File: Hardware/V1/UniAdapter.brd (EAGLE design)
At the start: 40 x 20.9 mm, 19 parts, among them IC1 LD1117S33TR, U1 STM32F072CBT6, U2 SN65HVD232D, X1 CAN Bus

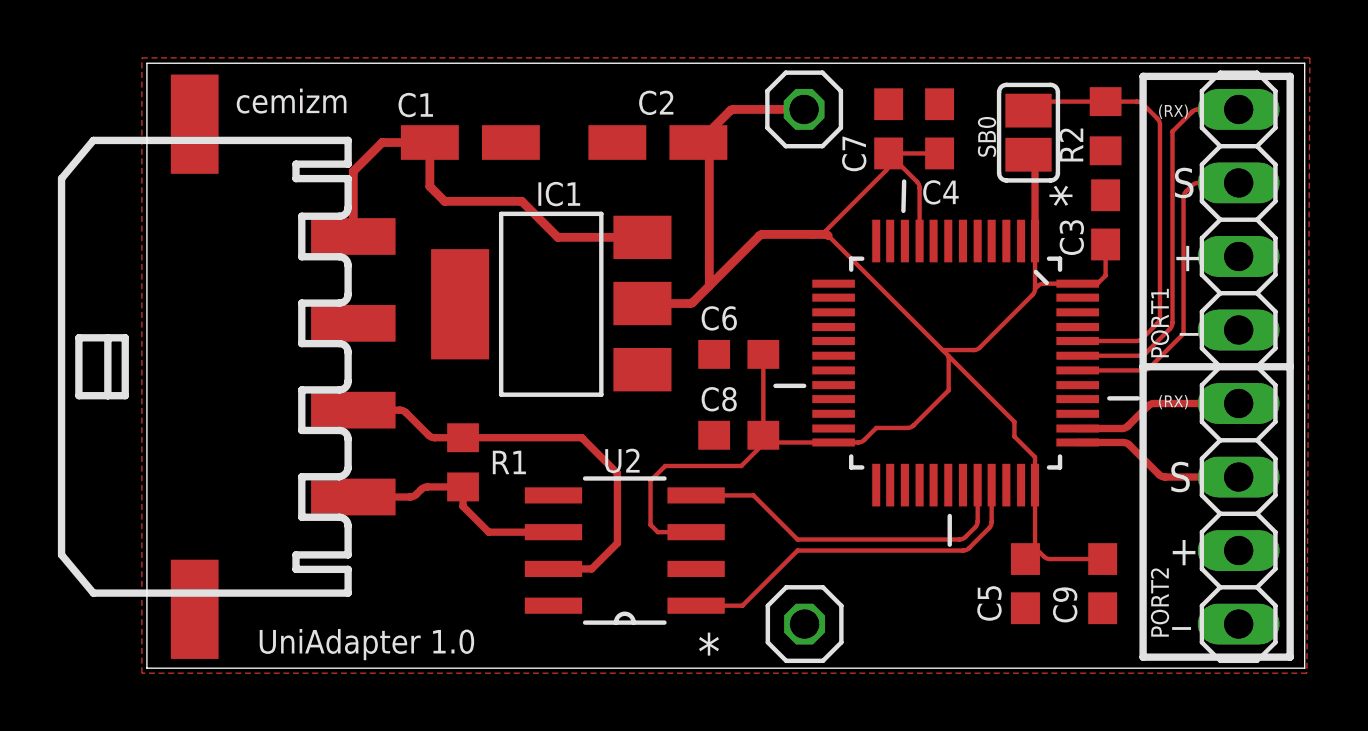
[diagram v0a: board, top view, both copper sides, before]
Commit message: [HW] UniAdapter 1.1
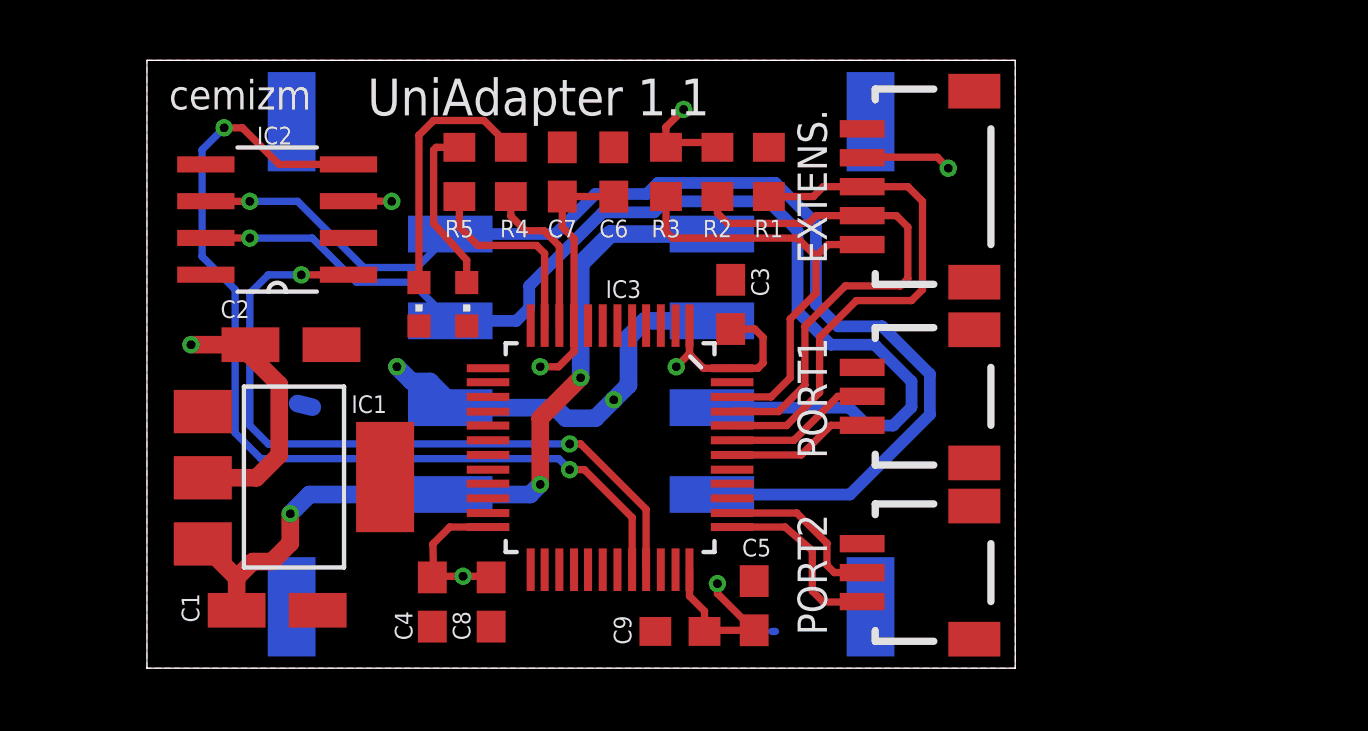
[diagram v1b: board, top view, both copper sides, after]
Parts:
- removed JP1: (no value), pinhead:1X08
- removed JP2, JP3: (no value), pinhead:1X01
- removed SB0: (no value), jumper:SJ
- removed U1: STM32F072CBT6, STM32F0:QFP50P900X900X160-48N
- removed U2: SN65HVD232D, texas:SOIC127P600X175-8N
- added EXTENS.: SM05B-SRSS-TB, con-jst2:SM05B-SRSS-TB
- added IC2: SN65HVD232D, texas:SOIC127P600X175-8N
- added IC3: STM32F072CBT6, STM32F0:LQFP48
- added LED_GREEN, LED_RED: (no value), led:CHIPLED_0603
- added PORT1, PORT2: SM03B-SRSS-TB, con-jst2:SM03B-SRSS-TB
- added R3: 1.8K, rcl:R0603
- added R4, R5: 55Ohm, rcl:R0603
- added X2: CAN Bus, con-molex-micro-fit-3_0:43650-0412
- C4: value 10nF -> 100nF
- C6: value 100nF -> 10nF
- R1: value 120 Ohm -> 10k
- R2: value 10k -> 1.8K
- moved C4 24.0 mm to (9.86, 2.29), turned to 270 degrees
- moved C1 17.5 mm to (4.50, 2.00)
- moved C9 14.7 mm to (18.4, 1.27), turned to 180 degrees
- moved R1 14.6 mm to (21.5, 17.1)
- moved C2 14.5 mm to (4.98, 11.2), turned to 0 degrees
- moved R2 13.5 mm to (19.7, 17.1)
- moved C3 13.3 mm to (20.2, 12.6)
- moved C7 11.4 mm to (14.4, 17.1)
- moved IC1 10.7 mm to (5.08, 6.60), turned to 270 degrees
- moved C8 10.3 mm to (11.9, 2.29), turned to 270 degrees
- moved C5 9.40 mm to (21.0, 2.16), turned to 90 degrees
- moved C6 7.64 mm to (16.1, 17.1), turned to 90 degrees
- moved X1 3.35 mm to (5.00, 10.5), flipped to the bottom, turned to 90 degrees
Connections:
- removed net NC1: JP1.3
- removed net NC2: JP1.7
- new net I2C1_SCL: EXTENS..2, IC3.45, R2.2
- new net I2C1_SDA: EXTENS..1, IC3.46, R3.2
- new net LD_GREEN: IC3.11, R5.1
- new net LD_RED: IC3.10, R4.1
- new net N$3: LED_RED.A, R4.2
- new net N$4: LED_GREEN.A, R5.2
- net 6V: now also X2.P$4
- net BOOT0: now also EXTENS..3, IC3.44, R1.1; no longer R2.1, SB0.1, U1.44
- net CANRX: now also IC2.4, IC3.32; no longer U1.32, U2.4
- net CANTX: now also IC2.1, IC3.33; no longer U1.33, U2.1
- net CAN_H: now also IC2.7, X2.P$2; no longer R1.2, U2.7
- net CAN_L: now also IC2.6, X2.P$1; no longer R1.1, U2.6
- net GND: now also EXTENS..5, IC2.2, IC3.23, IC3.35, IC3.47, IC3.8, LED_GREEN.C, LED_RED.C, PORT1.3, PORT2.3, R1.2, X2.P$3; no longer JP1.4, JP1.8, JP3.1, R2.2, U1.23, U1.35, U1.47, U1.8, U2.2
- net USART1RX: now also IC3.43, PORT1.2; no longer JP1.1, U1.43
- net USART1TX: now also IC3.42, PORT1.1; no longer JP1.2, U1.42
- net USART2RX: now also IC3.38, PORT2.2; no longer JP1.5, U1.38
- net USART2TX: now also IC3.37, PORT2.1; no longer JP1.6, U1.37
- net VCC: now also EXTENS..4, IC2.3, IC3.1, IC3.24, IC3.36, IC3.48, IC3.9, R2.1, R3.1; no longer JP2.1, SB0.2, U1.1, U1.24, U1.36, U1.48, U1.9, U2.3
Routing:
- net CAN_L: track 8.06 -> 41.6 mm, vias 0 -> 1
- net VCC: track 74.3 -> 46.1 mm, vias 0 -> 8
- net CAN_H: track 15.0 -> 40.2 mm, vias 0 -> 1
- net CANRX: track 11.9 -> 32.9 mm, vias 0 -> 2
- net I2C1_SCL: track 0.00 -> 18.5 mm
- net I2C1_SDA: track 0.00 -> 15.4 mm
- net GND: track 0.00 -> 14.1 mm, vias 0 -> 2
- net 6V: track 14.9 -> 28.4 mm, vias 0 -> 3
- net CANTX: track 12.7 -> 25.2 mm, vias 0 -> 2
- net N$3: track 0.00 -> 8.86 mm
- net USART1RX: track 13.0 -> 5.12 mm
- net LD_GREEN: track 0.00 -> 6.87 mm
- net USART1TX: track 11.0 -> 4.92 mm
- net N$4: track 0.00 -> 5.95 mm
- net LD_RED: track 0.00 -> 5.52 mm
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- added copper zone on layer 16, net VCC
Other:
- board size 40 x 20.9 mm -> 30 x 21 mm
- board text added: "UniAdapter 1.1"
- board text removed: "(RX)"
- board text removed: "+"
- board text removed: "PORT1"
- board text removed: "PORT2"
- board text removed: "S"
- board text removed: "UniAdapter 1.0"
- board text removed: "_"
